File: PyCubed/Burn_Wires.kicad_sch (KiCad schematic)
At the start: 4 parts, among them J19 F3311A7H121014E200, J4 1985807

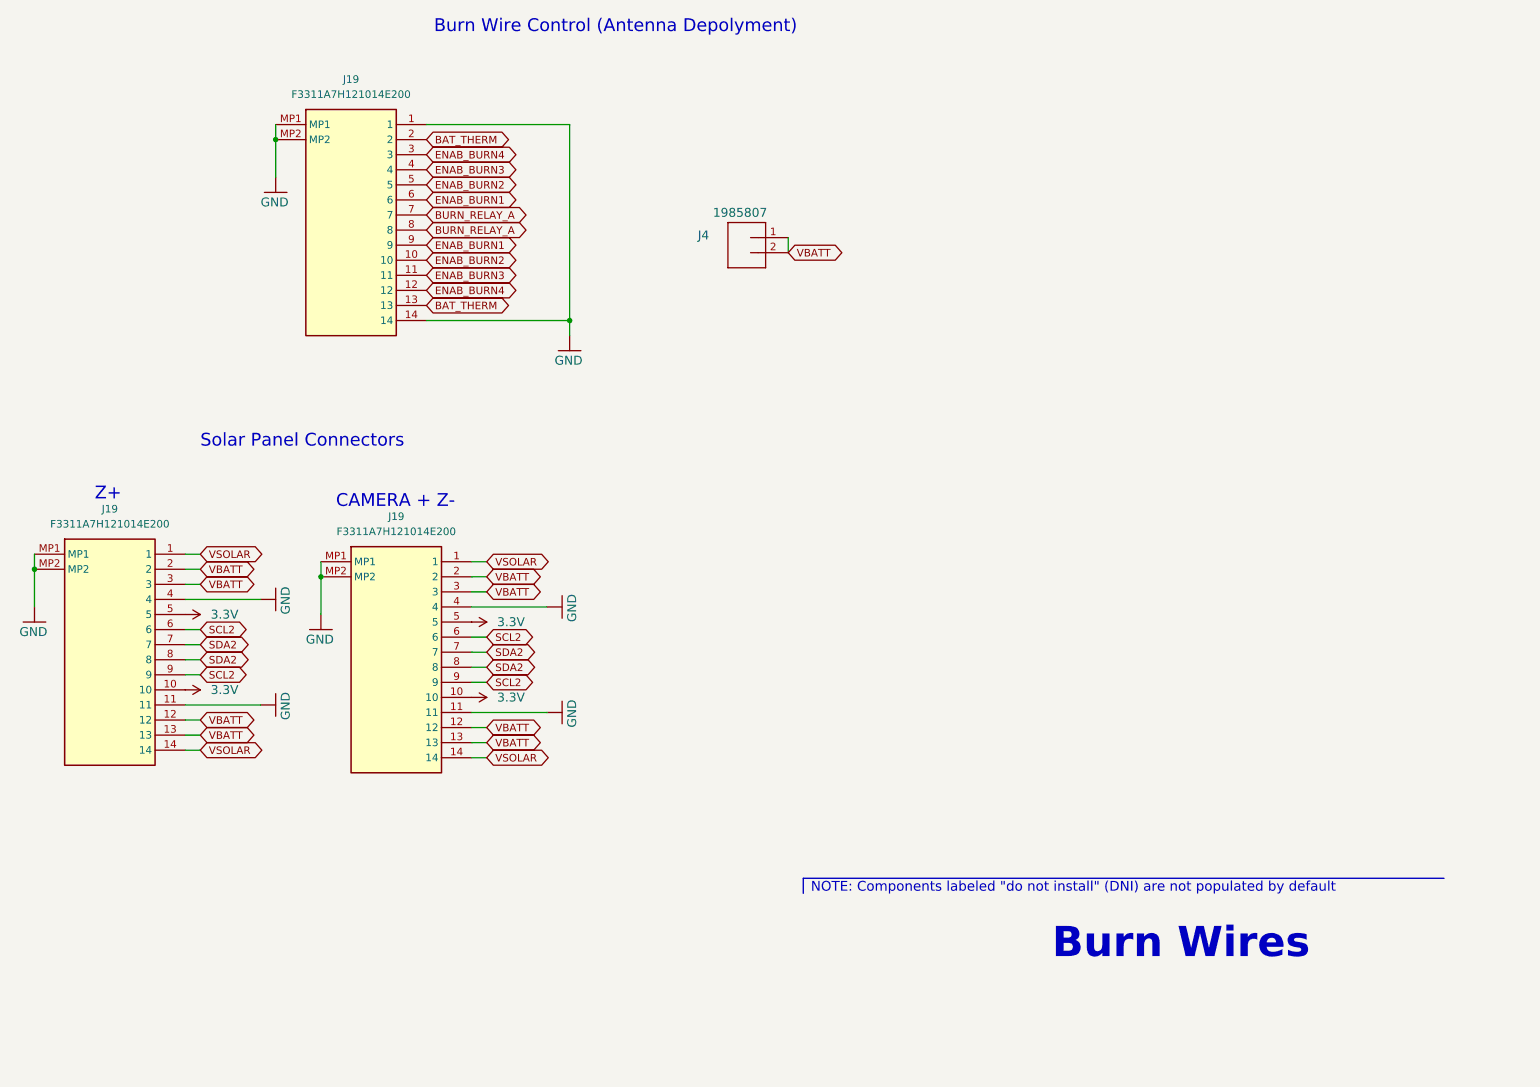
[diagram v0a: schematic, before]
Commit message: PyCubed Schematic Finalized
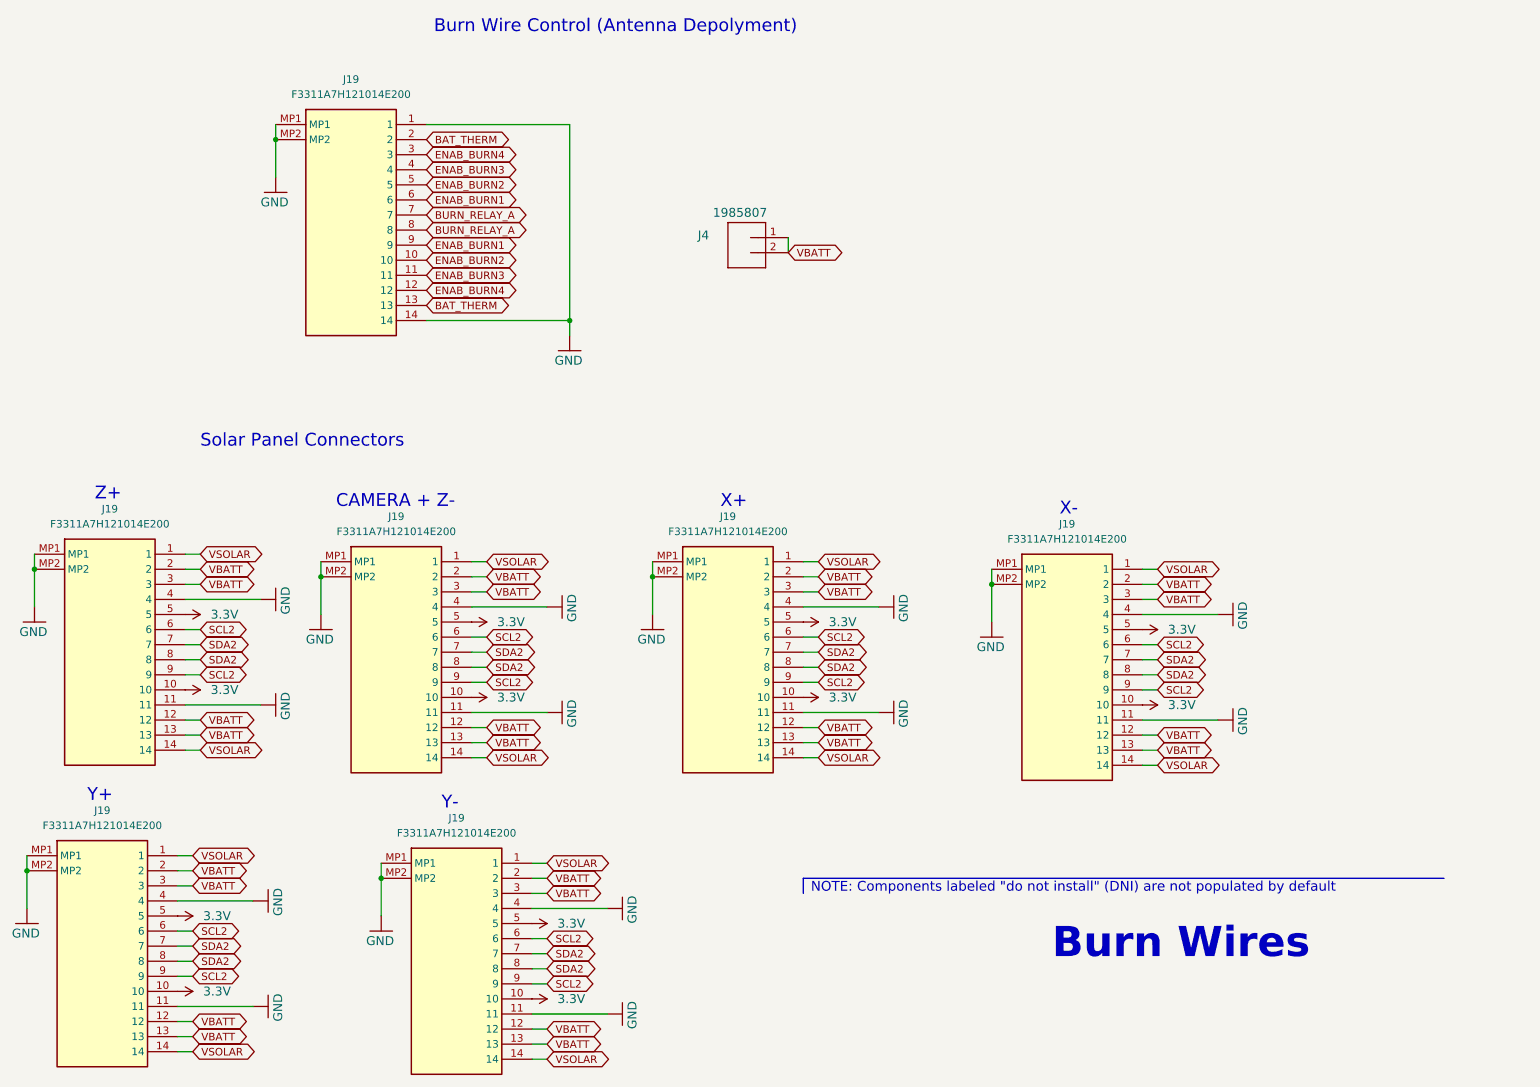
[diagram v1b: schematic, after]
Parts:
- added J19 (x4): F3311A7H121014E200, F3311A7H121014E200, symbol SamacSys_Parts:F3311A7H121014E200
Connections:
- net 3.3V: now also J19.10, J19.10, J19.10, J19.10, J19.5, J19.5, J19.5, J19.5
- net GND: now also J19.11, J19.11, J19.11, J19.11, J19.4, J19.4, J19.4, J19.4, J19.MP1, J19.MP1, J19.MP1, J19.MP1, J19.MP2, J19.MP2, J19.MP2, J19.MP2
- net SCL2: now also J19.6, J19.6, J19.6, J19.6, J19.9, J19.9, J19.9, J19.9
- net SDA2: now also J19.7, J19.7, J19.7, J19.7, J19.8, J19.8, J19.8, J19.8
- net VBATT: now also J19.12, J19.12, J19.12, J19.12, J19.13, J19.13, J19.13, J19.13, J19.2, J19.2, J19.2, J19.2, J19.3, J19.3, J19.3, J19.3
- net VSOLAR: now also J19.1, J19.1, J19.1, J19.1, J19.14, J19.14, J19.14, J19.14
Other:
- note added: "X+"
- note added: "X-"
- note added: "Y+"
- note added: "Y-"
